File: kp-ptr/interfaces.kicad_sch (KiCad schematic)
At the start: 19 parts, among them IC1 E22-900M22S, J11 u.fl, J4 USB_C_Receptacle_USB2.0, U10 USBLC6-2SC6, U11 W25Q128JVS, U2 NL27WZU04DBVT1G

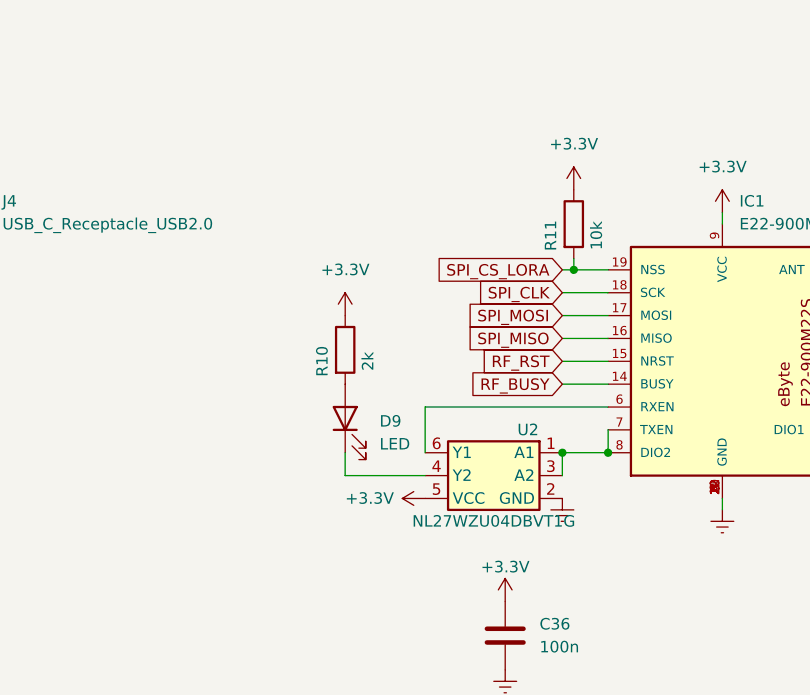
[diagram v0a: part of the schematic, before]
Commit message: Szlifowanie schematu
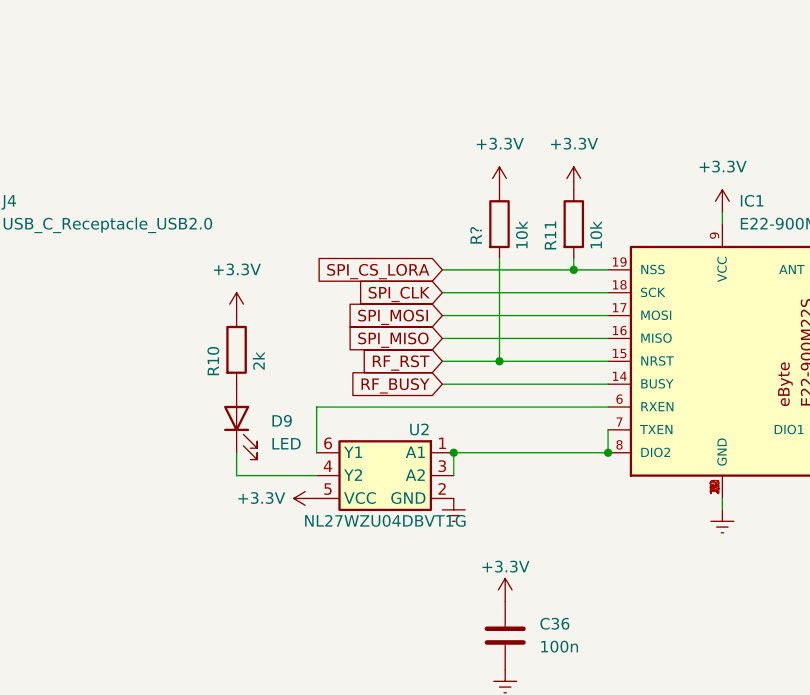
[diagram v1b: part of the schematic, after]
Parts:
- added R?: 10k, Resistor_SMD:R_0402_1005Metric_Pad0.72x0.64mm_HandSolder, symbol Device:R
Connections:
- net +3V3: now also R?.1
- net RF_RST: now also R?.2
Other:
- moved on the sheet: D9, R10, U2
